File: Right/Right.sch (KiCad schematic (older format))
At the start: 188 parts, among them SW0 SW_PUSH, SW1 SW_PUSH, SW10 SW_PUSH, SW100 SW_PUSH, SW1000 SW_Push_Dual_R, SW1001 SW_Push_Dual_R, SW1002 SW_Push_Dual_R, SW1003 SW_Push_Dual_R, SW1004 SW_Push_Dual_R, SW1005 SW_Push_Dual_R, SW101 SW_PUSH, SW102 SW_PUSH, SW103 SW_PUSH, SW104 SW_PUSH, SW105 SW_PUSH, SW106 SW_PUSH, SW11 SW_PUSH, SW110 SW_PUSH, SW111 SW_PUSH, SW112 SW_PUSH, SW113 SW_PUSH, SW114 SW_PUSH, SW115 SW_PUSH, SW116 SW_PUSH, SW12 SW_PUSH, SW13 SW_PUSH, SW14 SW_PUSH, SW15 SW_PUSH, SW2 SW_PUSH, SW20 SW_PUSH, SW21 SW_PUSH, SW22 SW_PUSH, SW23 SW_PUSH, SW24 SW_PUSH, SW25 SW_PUSH, SW3 SW_PUSH, SW30 SW_PUSH, SW31 SW_PUSH, SW32 SW_PUSH, SW33 SW_PUSH, SW34 SW_PUSH, SW35 SW_PUSH, SW4 SW_PUSH, SW40 SW_PUSH, SW41 SW_PUSH, SW42 SW_PUSH, SW43 SW_PUSH, SW44 SW_PUSH, SW45 SW_PUSH, SW5 SW_PUSH, SW50 SW_PUSH, SW51 SW_PUSH, SW52 SW_PUSH, SW53 SW_PUSH, SW54 SW_PUSH, SW60 SW_PUSH, SW61 SW_PUSH, SW62 SW_PUSH, SW63 SW_PUSH, SW64 SW_PUSH, SW65 SW_PUSH, SW66 SW_PUSH, SW70 SW_PUSH, SW71 SW_PUSH, SW72 SW_PUSH, SW73 SW_PUSH, SW74 SW_PUSH, SW75 SW_PUSH, SW76 SW_PUSH, SW77 SW_PUSH, SW80 SW_PUSH, SW81 SW_PUSH, SW82 SW_PUSH, SW83 SW_PUSH, SW84 SW_PUSH, SW85 SW_PUSH, SW86 SW_PUSH, SW87 SW_PUSH, SW90 SW_PUSH, SW91 SW_PUSH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

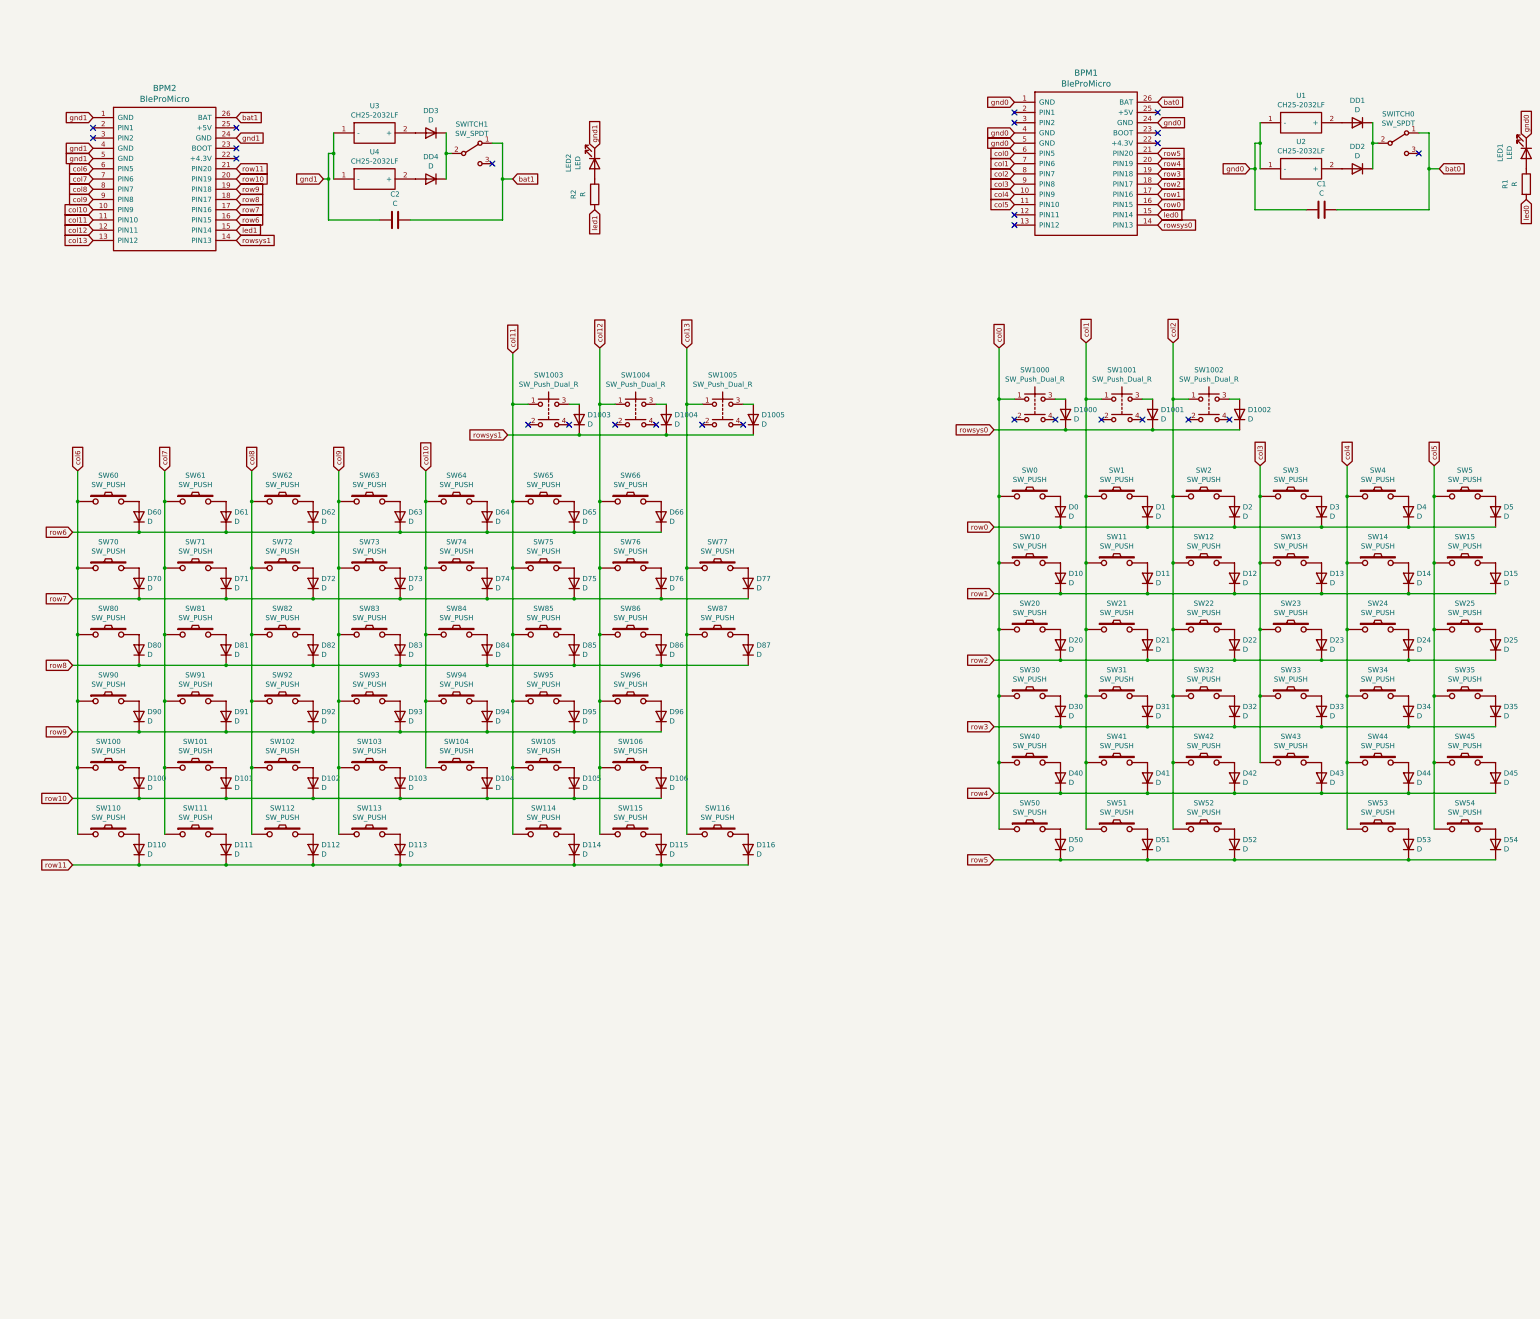
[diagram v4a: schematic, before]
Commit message: 途中
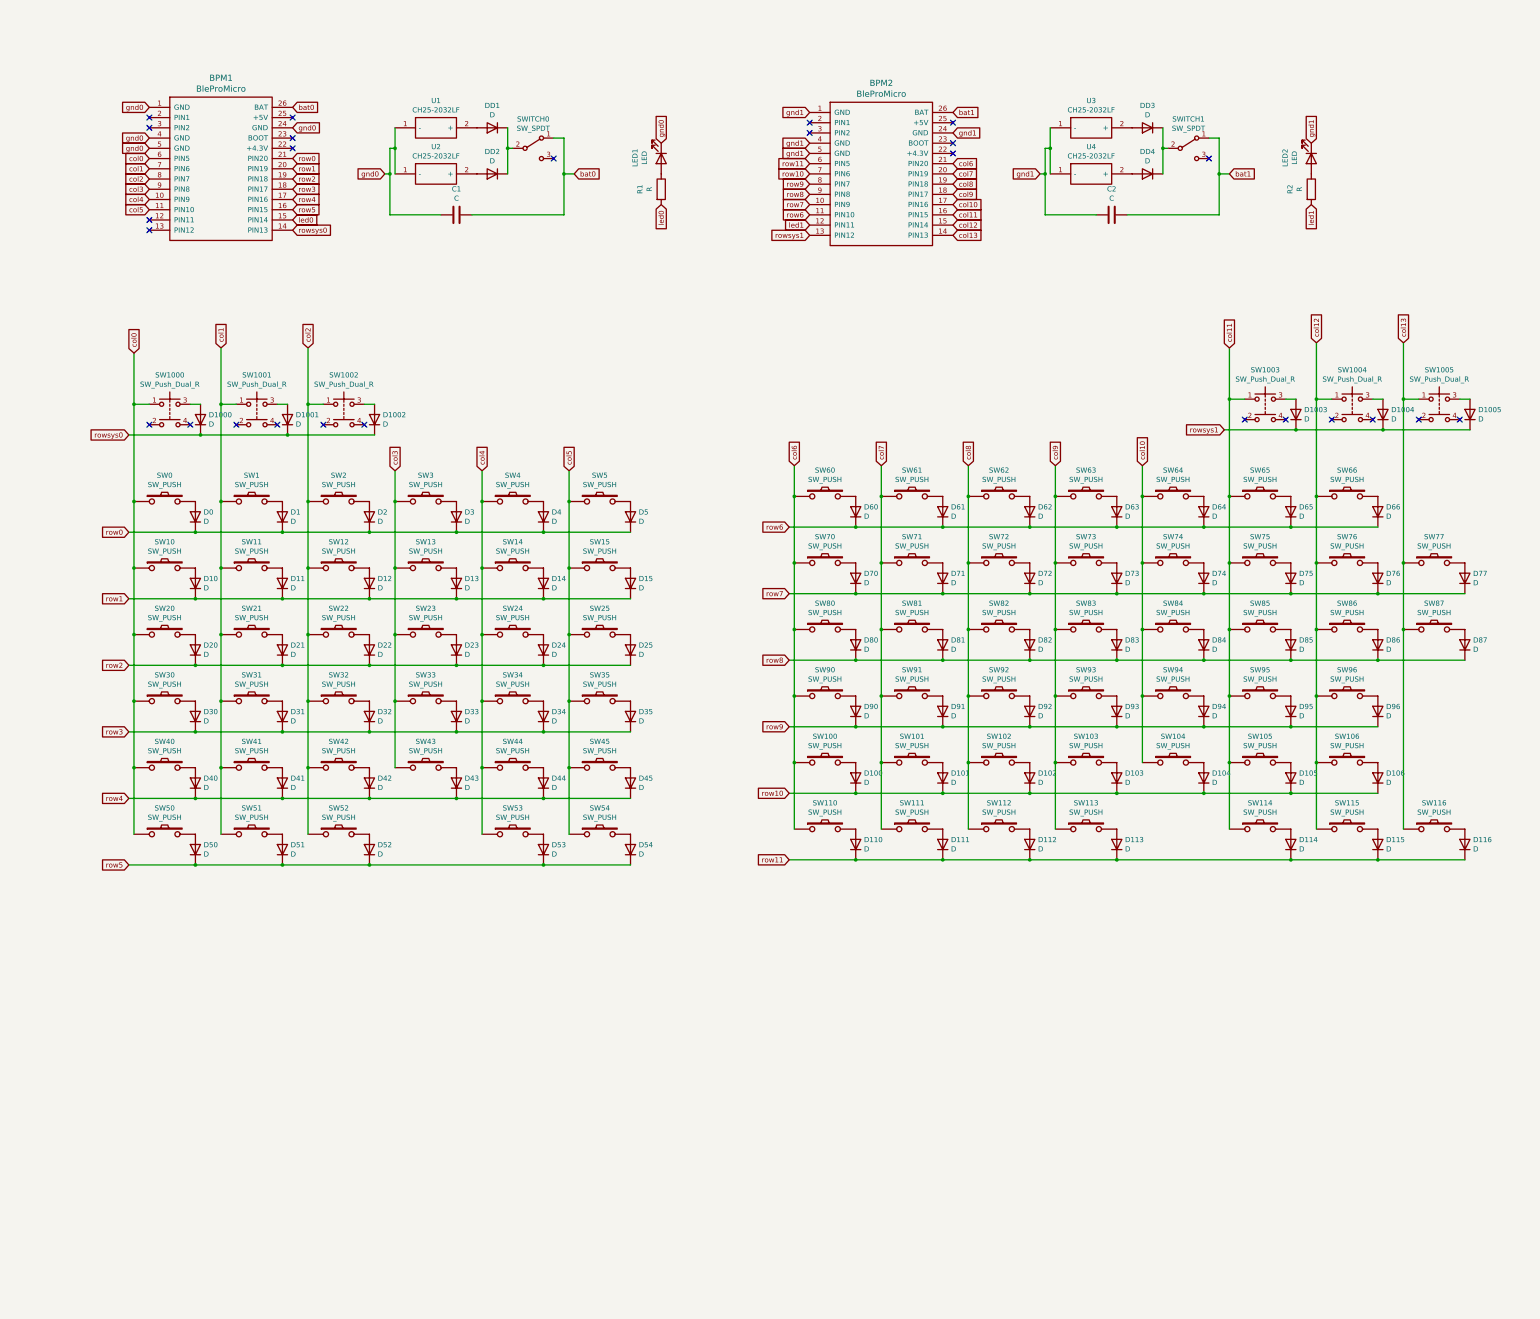
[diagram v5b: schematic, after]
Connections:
- net col10: now also BPM2.17 (PIN16); no longer BPM2.10 (PIN9)
- net col11: now also BPM2.16 (PIN15); no longer BPM2.11 (PIN10)
- net col12: now also BPM2.15 (PIN14); no longer BPM2.12 (PIN11)
- net col13: now also BPM2.14 (PIN13); no longer BPM2.13 (PIN12)
- net col6: now also BPM2.21 (PIN20); no longer BPM2.6 (PIN5)
- net col7: now also BPM2.20 (PIN19); no longer BPM2.7 (PIN6)
- net col8: now also BPM2.19 (PIN18); no longer BPM2.8 (PIN7)
- net col9: now also BPM2.18 (PIN17); no longer BPM2.9 (PIN8)
- net led1: now also BPM2.12 (PIN11); no longer BPM2.15 (PIN14)
- net row0: now also BPM1.21 (PIN20); no longer BPM1.16 (PIN15)
- net row1: now also BPM1.20 (PIN19); no longer BPM1.17 (PIN16)
- net row10: now also BPM2.7 (PIN6); no longer BPM2.20 (PIN19)
- net row11: now also BPM2.6 (PIN5); no longer BPM2.21 (PIN20)
- net row2: now also BPM1.19 (PIN18); no longer BPM1.18 (PIN17)
- net row3: now also BPM1.18 (PIN17); no longer BPM1.19 (PIN18)
- net row4: now also BPM1.17 (PIN16); no longer BPM1.20 (PIN19)
- net row5: now also BPM1.16 (PIN15); no longer BPM1.21 (PIN20)
- net row6: now also BPM2.11 (PIN10); no longer BPM2.16 (PIN15)
- net row7: now also BPM2.10 (PIN9); no longer BPM2.17 (PIN16)
- net row8: now also BPM2.9 (PIN8); no longer BPM2.18 (PIN17)
- net row9: now also BPM2.8 (PIN7); no longer BPM2.19 (PIN18)
- net rowsys1: now also BPM2.13 (PIN12); no longer BPM2.14 (PIN13)
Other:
- moved on the sheet: BPM1, BPM2, C1, C2, D0, D1, D10, D100, D1000, D1001, D1002, D1003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

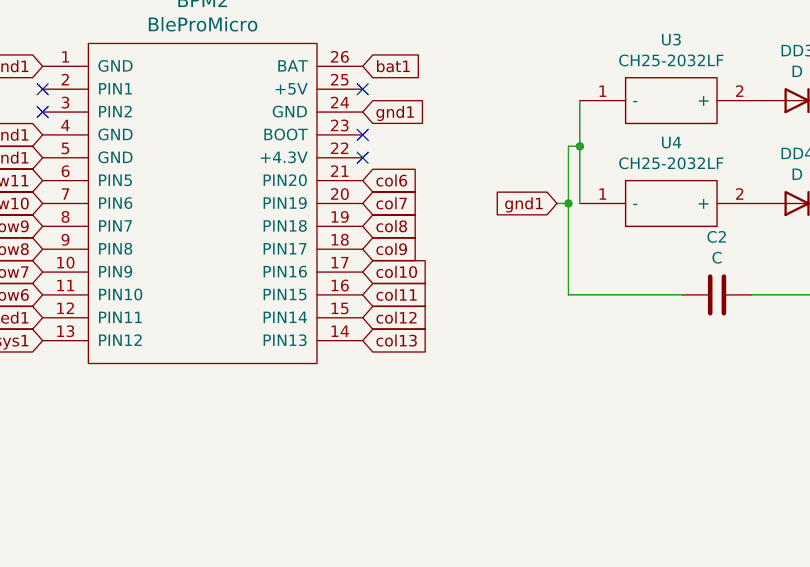
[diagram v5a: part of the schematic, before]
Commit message: とりあえず右手全部つながった
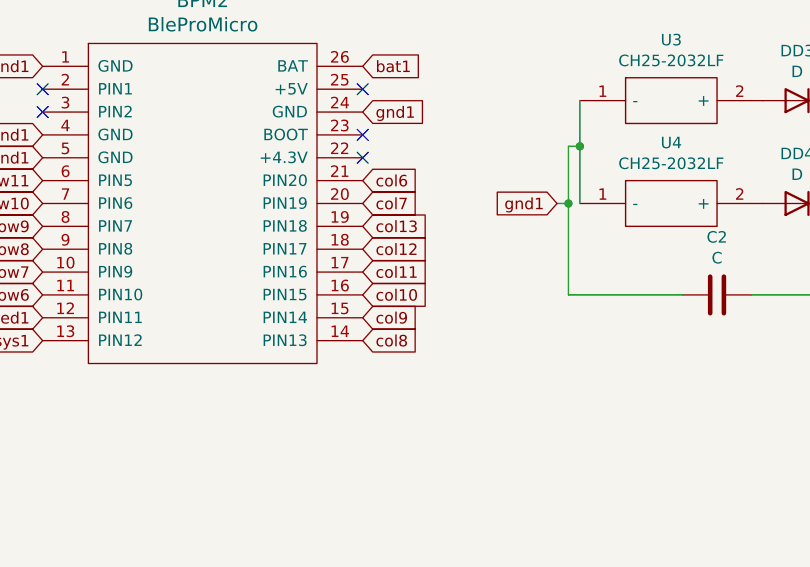
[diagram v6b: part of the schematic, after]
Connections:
- net col10: now also BPM2.16 (PIN15); no longer BPM2.17 (PIN16)
- net col11: now also BPM2.17 (PIN16); no longer BPM2.16 (PIN15)
- net col12: now also BPM2.18 (PIN17); no longer BPM2.15 (PIN14)
- net col13: now also BPM2.19 (PIN18); no longer BPM2.14 (PIN13)
- net col8: now also BPM2.14 (PIN13); no longer BPM2.19 (PIN18)
- net col9: now also BPM2.15 (PIN14); no longer BPM2.18 (PIN17)
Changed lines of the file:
@@
 Text GLabel 9950 2500 2    50   Input ~ 0
 col7
+Text GLabel 9950 3100 2    50   Input ~ 0
+col8
+Text GLabel 9950 3000 2    50   Input ~ 0
+col9
+Text GLabel 9950 2900 2    50   Input ~ 0
+col10
+Text GLabel 9950 2800 2    50   Input ~ 0
+col11
+Text GLabel 9950 2700 2    50   Input ~ 0
+col12
 Text GLabel 9950 2600 2    50   Input ~ 0
-col8
-Text GLabel 9950 2700 2    50   Input ~ 0
-col9
-Text GLabel 9950 2800 2    50   Input ~ 0
-col10
-Text GLabel 9950 2900 2    50   Input ~ 0
-col11
-Text GLabel 9950 3000 2    50   Input ~ 0
-col12
-Text GLabel 9950 3100 2    50   Input ~ 0
 col13
 $EndSCHEMATC

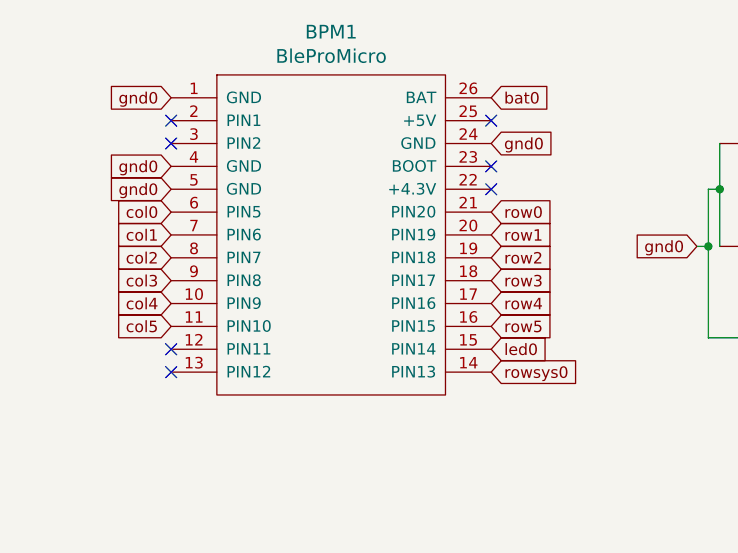
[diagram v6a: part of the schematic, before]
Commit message: 左手導線
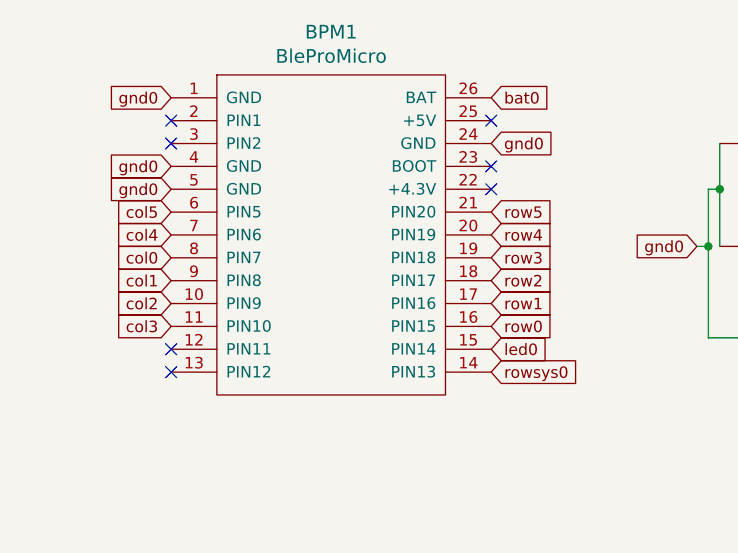
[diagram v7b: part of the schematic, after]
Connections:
- net col0: now also BPM1.8 (PIN7); no longer BPM1.6 (PIN5)
- net col1: now also BPM1.9 (PIN8); no longer BPM1.7 (PIN6)
- net col2: now also BPM1.10 (PIN9); no longer BPM1.8 (PIN7)
- net col3: now also BPM1.11 (PIN10); no longer BPM1.9 (PIN8)
- net col4: now also BPM1.7 (PIN6); no longer BPM1.10 (PIN9)
- net col5: now also BPM1.6 (PIN5); no longer BPM1.11 (PIN10)
- net row0: now also BPM1.16 (PIN15); no longer BPM1.21 (PIN20)
- net row1: now also BPM1.17 (PIN16); no longer BPM1.20 (PIN19)
- net row2: now also BPM1.18 (PIN17); no longer BPM1.19 (PIN18)
- net row3: now also BPM1.19 (PIN18); no longer BPM1.18 (PIN17)
- net row4: now also BPM1.20 (PIN19); no longer BPM1.17 (PIN16)
- net row5: now also BPM1.21 (PIN20); no longer BPM1.16 (PIN15)
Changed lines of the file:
@@
 NoConn ~ 2100 3050
 NoConn ~ 2100 2950
+Text GLabel 2100 2350 0    50   Input ~ 0
+col5
+Text GLabel 2100 2450 0    50   Input ~ 0
+col4
 Text GLabel 2100 2850 0    50   Input ~ 0
-col5
+col3
 Text GLabel 2100 2750 0    50   Input ~ 0
-col4
+col2
 Text GLabel 2100 2650 0    50   Input ~ 0
-col3
+col1
 Text GLabel 2100 2550 0    50   Input ~ 0
-col2
-Text GLabel 2100 2450 0    50   Input ~ 0
-col1
-Text GLabel 2100 2350 0    50   Input ~ 0
 col0
+Text GLabel 3500 2850 2    50   Input ~ 0
+row0
+Text GLabel 3500 2750 2    50   Input ~ 0
+row1
+Text GLabel 3500 2650 2    50   Input ~ 0
+row2
+Text GLabel 3500 2550 2    50   Input ~ 0
+row3
+Text GLabel 3500 2450 2    50   Input ~ 0
+row4
 Text GLabel 3500 2350 2    50   Input ~ 0
-row0
-Text GLabel 3500 2450 2    50   Input ~ 0
-row1
-Text GLabel 3500 2550 2    50   Input ~ 0
-row2
-Text GLabel 3500 2650 2    50   Input ~ 0
-row3
-Text GLabel 3500 2750 2    50   Input ~ 0
-row4
-Text GLabel 3500 2850 2    50   Input ~ 0
 row5
 Text GLabel 8550 3000 0    50   Input ~ 0
